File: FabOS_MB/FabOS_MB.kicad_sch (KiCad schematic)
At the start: 4 parts, among them J1 USB_A, U1 STM32F407VETx, U3 NCV7329, U5 HF3F-L 12-1ZL1T

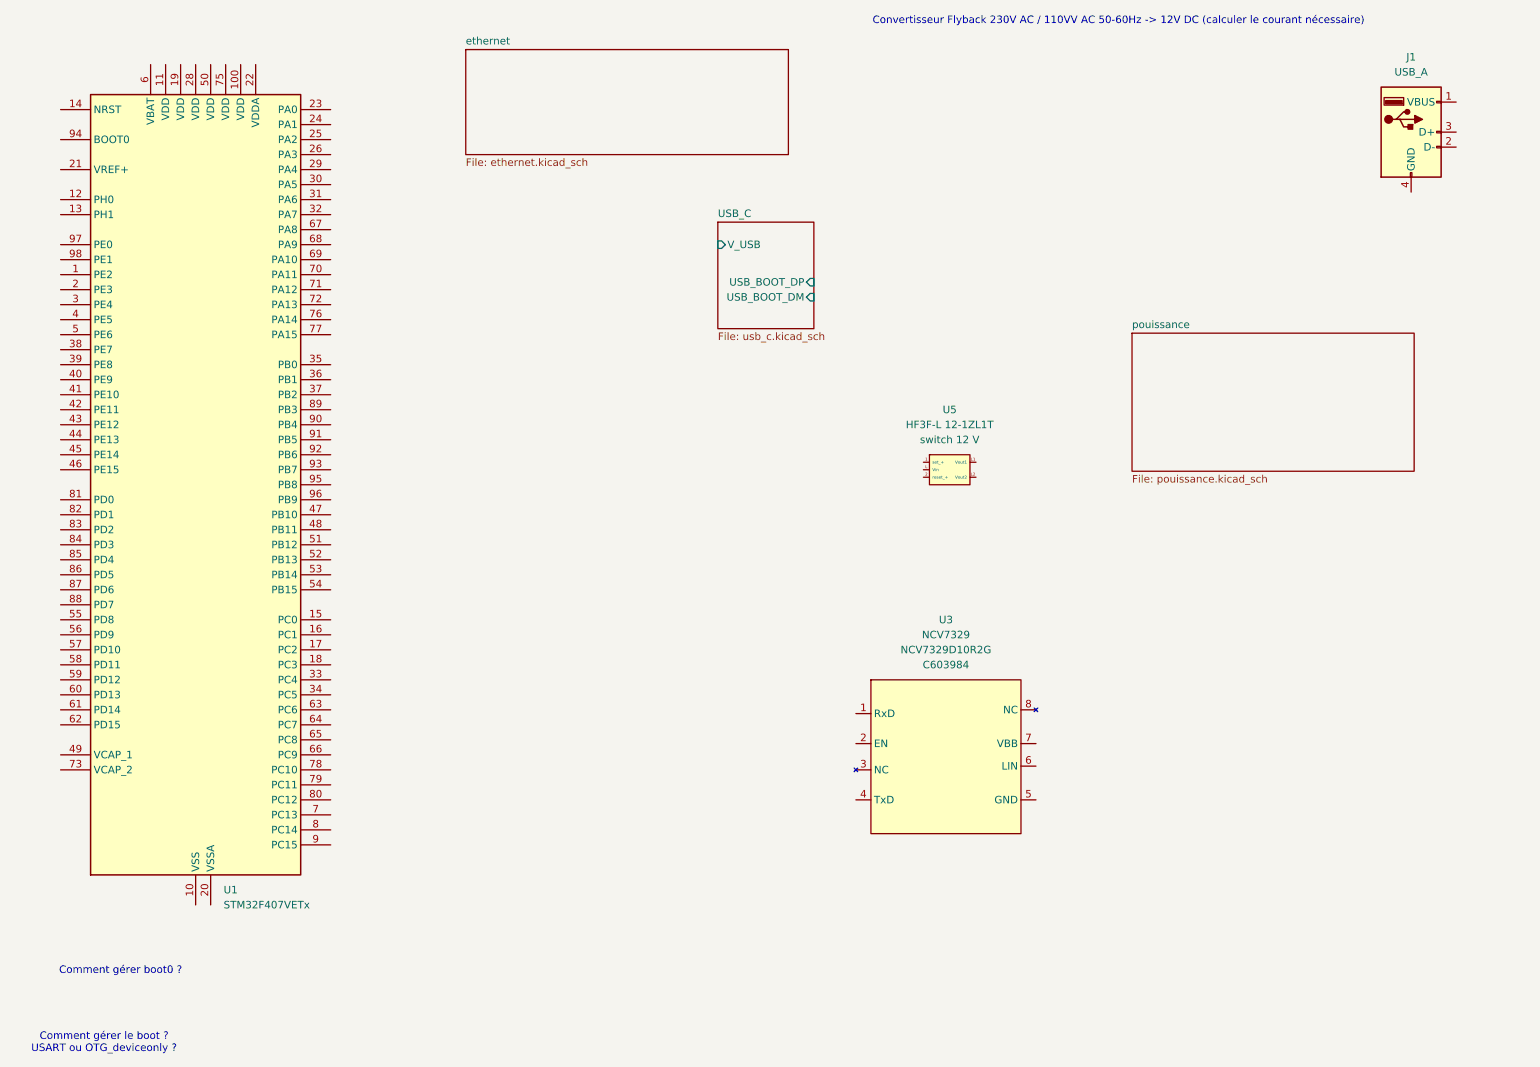
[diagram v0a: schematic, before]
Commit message: Début LIN
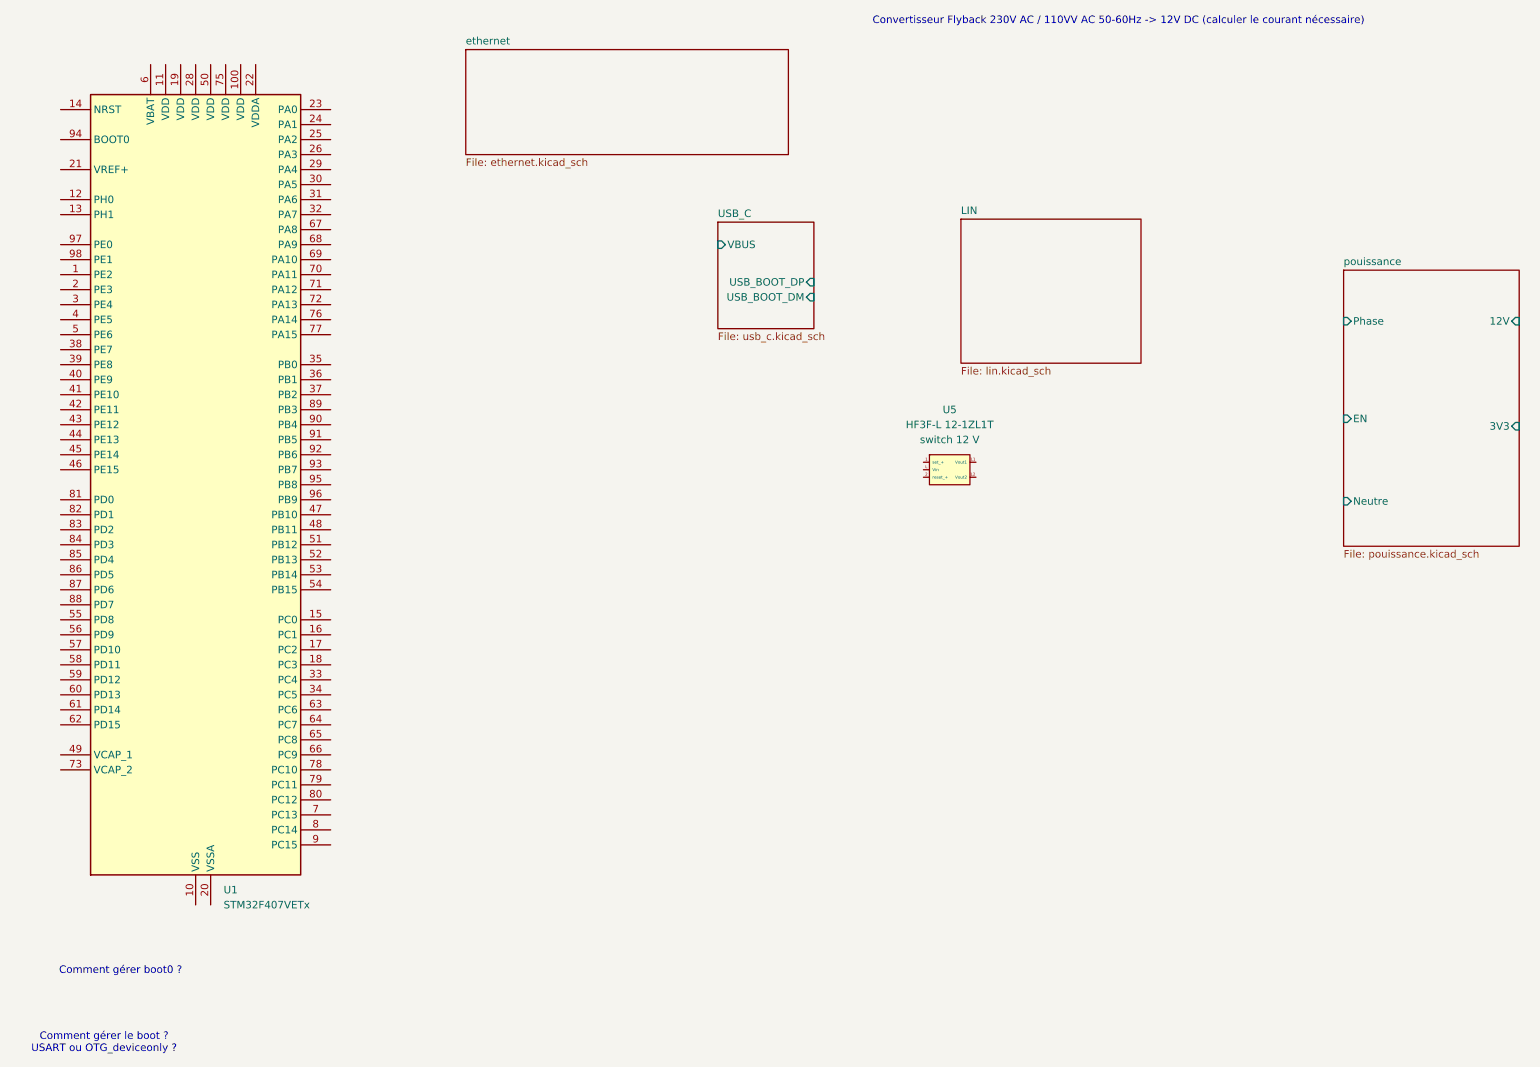
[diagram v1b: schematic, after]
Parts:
- removed J1: USB_A, Librairie_MB:USB_A_Femelle, symbol Connector:USB_A
- removed U3: NCV7329, Librairie_MB:NCV7329, symbol Librairie_MB:NCV7329
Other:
- added sheet LIN (lin.kicad_sch)
- sheet USB_C ports: added VBUS; removed V_USB
- sheet pouissance ports: added 12V, 3V3, EN, Neutre, Phase; removed none
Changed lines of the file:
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@@
-		)
-	)
-	(symbol
-		(lib_id "Librairie_MB:NCV7329")
-		(at 176.53 143.51 0)
-		(unit 1)
-		(exclude_from_sim no)
-		(in_bom yes)
-		(on_board yes)
-		(dnp no)
-		(fields_autoplaced yes)
-		(property "Reference" "U3"
-			(at 176.53 120.65 0)
-			(effects
-				(font
-					(size 1.27 1.27)
-				)
-			)
-		)
-		(property "Value" "NCV7329"
-			(at 176.53 123.19 0)
-			(effects
-				(font
-					(size 1.27 1.27)
-				)
-			)
-		)
-		(property "Footprint" "Librairie_MB:NCV7329"
-			(at 176.53 143.51 0)
-			(effects
-				(font
-					(size 1.27 1.27)
-				)
-				(hide yes)
-			)
-		)
-		(property "Datasheet" "https://www.lcsc.com/datasheet/lcsc_datasheet_2210210000_onsemi-NCV7329D10R2G_C603984.pdf"
-			(at 176.53 129.54 0)
-			(effects
-				(font
-					(size 1.27 1.27)
-				)
-				(hide yes)
-			)
-		)
-		(property "Description" "LIN Trans/receiver"
-			(at 176.53 127.635 0)
-			(effects
-				(font
-					(size 1.27 1.27)
-				)
-				(hide yes)
-			)
-		)
-		(property "MPN" "NCV7329D10R2G"
-			(at 176.53 125.73 0)
-			(effects
-				(font
-					(size 1.27 1.27)
-				)
-			)
-		)
-		(property "LCSC" "C603984 "
-			(at 176.53 128.27 0)
-			(effects
-				(font
-					(size 1.27 1.27)
-				)
-			)
-		)
-		(pin "3"
-		)
-		(pin "2"
-		)
-		(pin "1"
-		)
-		(pin "8"
-		)
-		(pin "4"
-		)
-		(pin "5"
-		)
-		(pin "7"
-		)
-		(pin "6"
-		)
-		(instances
-			(project ""
-				(path "/09377d5d-727f-4ff4-92c8-7a0483d23f1e"
-					(reference "U3")
-					(unit 1)
-				)
-			)
-		)
-	)
-	(symbol
-		(lib_id "Connector:USB_A")
-		(at 255.27 38.1 0)
-		(unit 1)
-		(exclude_from_sim no)
-		(in_bom yes)
-		(on_board yes)
-		(dnp no)
-		(fields_autoplaced yes)
-		(property "Reference" "J1"
-			(at 255.27 25.4 0)
-			(effects
-				(font
-					(size 1.27 1.27)
-				)
-			)
-		)
-		(property "Value" "USB_A"
-			(at 255.27 27.94 0)
-			(effects
-				(font
-					(size 1.27 1.27)
-				)
-			)
-		)
-		(property "Footprint" "Librairie_MB:USB_A_Femelle"
-			(at 259.08 39.37 0)
-			(effects
-				(font
-					(size 1.27 1.27)
-				)
-				(hide yes)
-			)
-		)
-		(property "Datasheet" "https://www.lcsc.com/datasheet/lcsc_datasheet_2103011233_Jing-Extension-of-the-Electronic-Co--908-371A1011D10100_C42576.pdf"
-			(at 259.08 39.37 0)
-			(effects
-				(font
-					(size 1.27 1.27)
-				)
-				(hide yes)
-			)
-		)
-		(property "Description" "USB Type A connector"
-			(at 255.27 38.1 0)
-			(effects
-				(font
-					(size 1.27 1.27)
-				)
-				(hide yes)
-			)
-		)
-		(property "MPN" "  908-371A1011D10100"
-			(at 255.27 38.1 0)
-			(effects
-				(font
-					(size 1.27 1.27)
-				)
-				(hide yes)
-			)
-		)
-		(property "LCSC" "  C42576"
-			(at 255.27 38.1 0)
-			(effects
-				(font
-					(size 1.27 1.27)
-				)
-				(hide yes)
-			)
-		)
-		(pin "2"
-		)
-		(pin "4"
-		)
-		(pin "1"
-		)
-		(pin "3"
-		)
-		(instances
-			(project ""
-				(path "/09377d5d-727f-4ff4-92c8-7a0483d23f1e"
-					(reference "J1")
-					(unit 1)
-				)
-			)
 		)
 	)
@@
 			)
 		)
-		(pin "V_USB" input
-			(at 137.922 57.15 180)
-			(effects
-				(font
-					(size 1.27 1.27)
-				)
-				(justify left)
-			)
-		)
 		(pin "USB_BOOT_DM" input
 			(at 154.178 66.04 0)
@@
 			)
 		)
+		(pin "VBUS" input
+			(at 137.922 57.15 180)
+			(effects
+				(font
+					(size 1.27 1.27)
+				)
+				(justify left)
+			)
+		)
 		(instances
 			(project "FabOS_MB"
@@
 	)
 	(sheet
-		(at 208.026 72.136)
-		(size 47.752 23.368)
+		(at 243.84 61.468)
+		(size 29.718 46.736)
 		(fields_autoplaced yes)
 		(stroke
@@
 		)
 		(property "Sheetname" "pouissance"
-			(at 208.026 71.4244 0)
+			(at 243.84 60.7564 0)
 			(effects
 				(font
@@
 		)
 		(property "Sheetfile" "pouissance.kicad_sch"
-			(at 208.026 96.0886 0)
-			(effects
-				(font
-					(size 1.27 1.27)
-				)
-				(justify left top)
+			(at 243.84 108.7886 0)
+			(effects
+				(font
+					(size 1.27 1.27)
+				)
+				(justify left top)
+			)
+		)
+		(pin "Neutre" input
+			(at 243.84 100.584 180)
+			(effects
+				(font
+					(size 1.27 1.27)
+				)
+				(justify left)
+			)
+		)
+		(pin "Phase" input
+			(at 243.84 70.104 180)
+			(effects
+				(font
+					(size 1.27 1.27)
+				)
+				(justify left)
+			)
+		)
+		(pin "12V" input
+			(at 273.558 70.104 0)
+			(effects
+				(font
+					(size 1.27 1.27)
+				)
+				(justify right)
+			)
+		)
+		(pin "EN" input
+			(at 243.84 86.614 180)
+			(effects
+				(font
+					(size 1.27 1.27)
+				)
+				(justify left)
+			)
+		)
+		(pin "3V3" input
+			(at 273.558 87.884 0)
+			(effects
+				(font
+					(size 1.27 1.27)
+				)
+				(justify right)
 			)
 		)
@@
 				)
 			)
+		)
+	)
+	(sheet
+		(at 179.07 52.832)
+		(size 30.48 24.384)
+		(fields_autoplaced yes)
+		(stroke
+			(width 0.1524)
+			(type solid)
+		)
+		(fill
+			(color 0 0 0 0.0000)
+		)
+		(property "Sheetname" "LIN"
+			(at 179.07 52.1204 0)
+			(effects
+				(font
+					(size 1.27 1.27)
+				)
+				(justify left bottom)
+			)
+		)
+		(property "Sheetfile" "lin.kicad_sch"
+			(at 179.07 77.8006 0)
+			(effects
+				(font
+					(size 1.27 1.27)
+				)
+				(justify left top)
+			)
+		)
+		(instances
+			(project "FabOS_MB"
+				(path "/09377d5d-727f-4ff4-92c8-7a0483d23f1e"
+					(page "5")
+				)
+			)
